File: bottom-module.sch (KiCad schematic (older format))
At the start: 15 parts, among them J10 Conn_02x12_Odd_Even, J13 PROTO1, J18 PROTO1, J5 Screw_Terminal_01x06, J6 Conn_02x12_Odd_Even, J8 Screw_Terminal_01x02, J9 Conn_02x12_Odd_Even

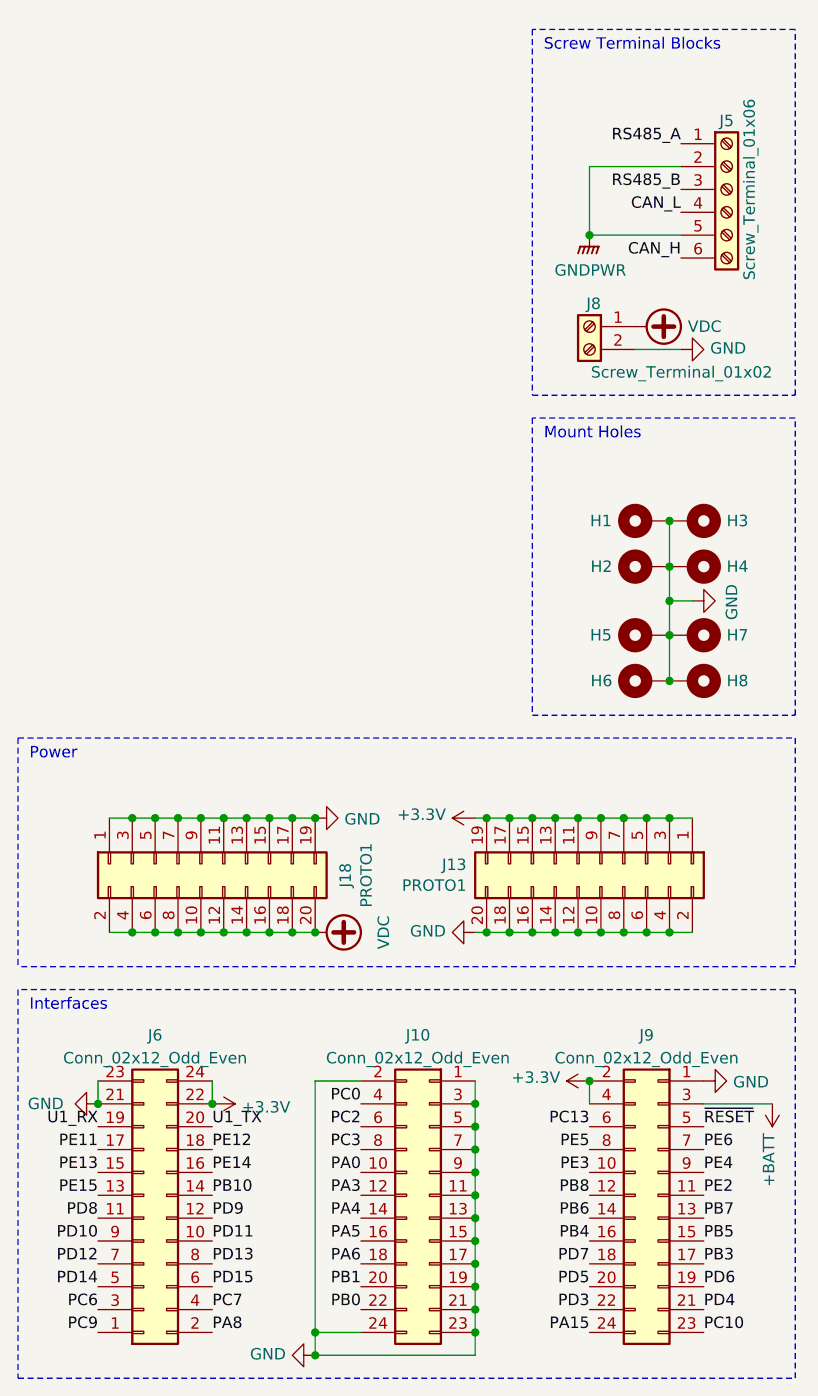
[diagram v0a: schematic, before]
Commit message: Clean module
Signed-off-by: Martin Ribelotta <martinribelotta@gmail.com>
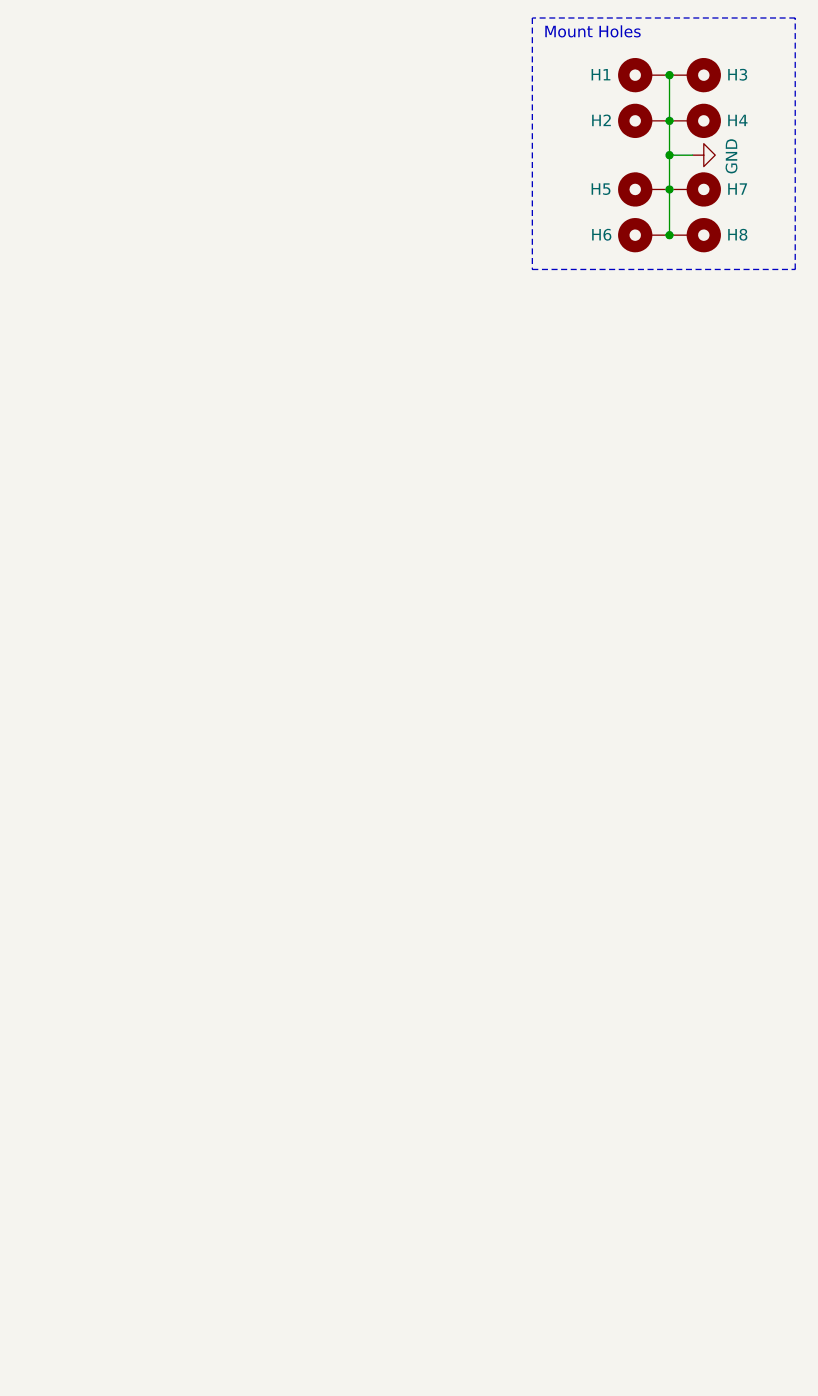
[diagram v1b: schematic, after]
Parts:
- removed J10, J6, J9: Conn_02x12_Odd_Even, Connector_PinSocket_2.54mm:PinSocket_2x12_P2.54mm_Vertical, symbol Connector_Generic:Conn_02x12_Odd_Even
- removed J13, J18: PROTO1, Connector_PinHeader_2.54mm:PinHeader_2x10_P2.54mm_Vertical, symbol Connector_Generic:Conn_02x10_Odd_Even
- removed J5: Screw_Terminal_01x06, Connectors_Phoenix:PhoenixContact_MC-G_06x5.08mm_Angled, symbol Connector:Screw_Terminal_01x06
- removed J8: Screw_Terminal_01x02, Connectors_Phoenix:PhoenixContact_MC-G_02x5.08mm_Angled, symbol Connector:Screw_Terminal_01x02
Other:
- note removed: "Interfaces"
- note removed: "Power"
- note removed: "Screw Terminal Blocks"
- moved on the sheet: H1, H2, H3, H4, H5, H6, H7, H8
